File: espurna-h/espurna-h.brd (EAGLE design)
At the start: 50 x 50 mm, 55 parts, among them IC1 AMS1117-3.3, IC2 ESP-12-SMD, IC4 HLW8012

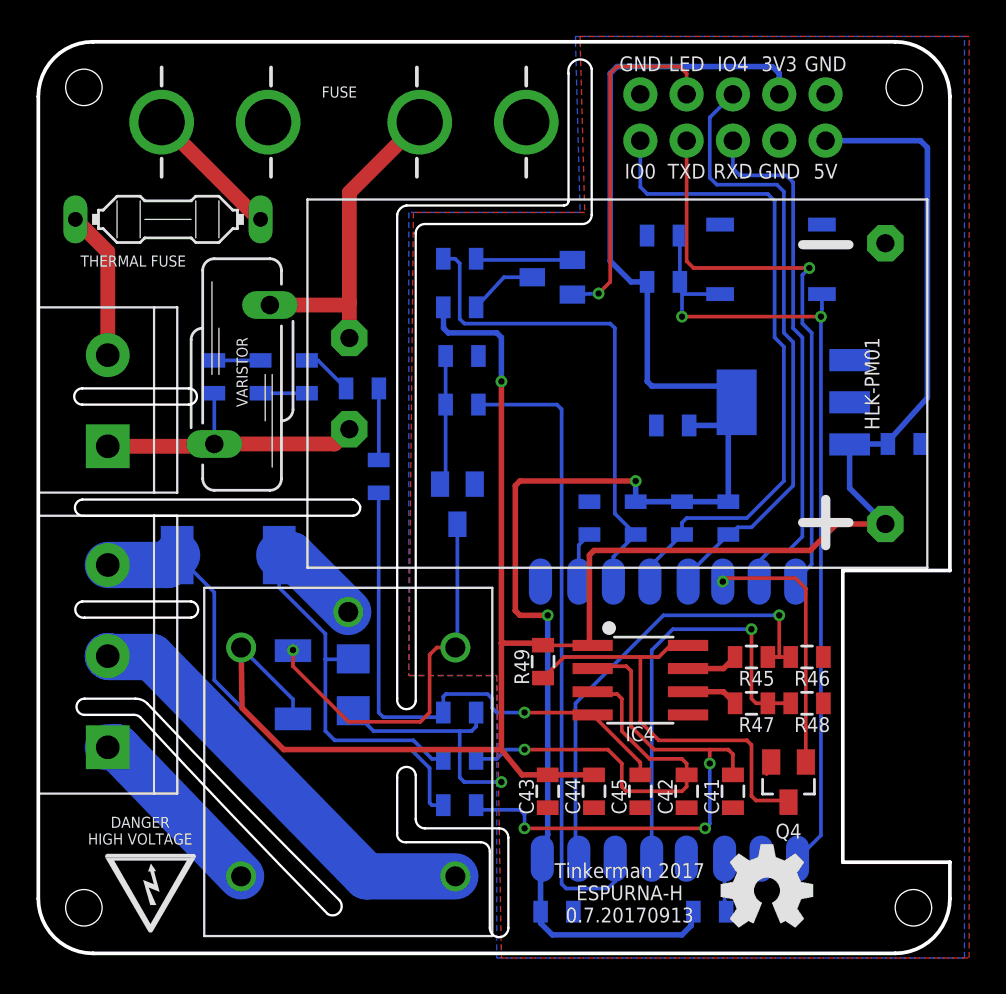
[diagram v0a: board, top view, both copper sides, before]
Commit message: Version 0.7.20170913
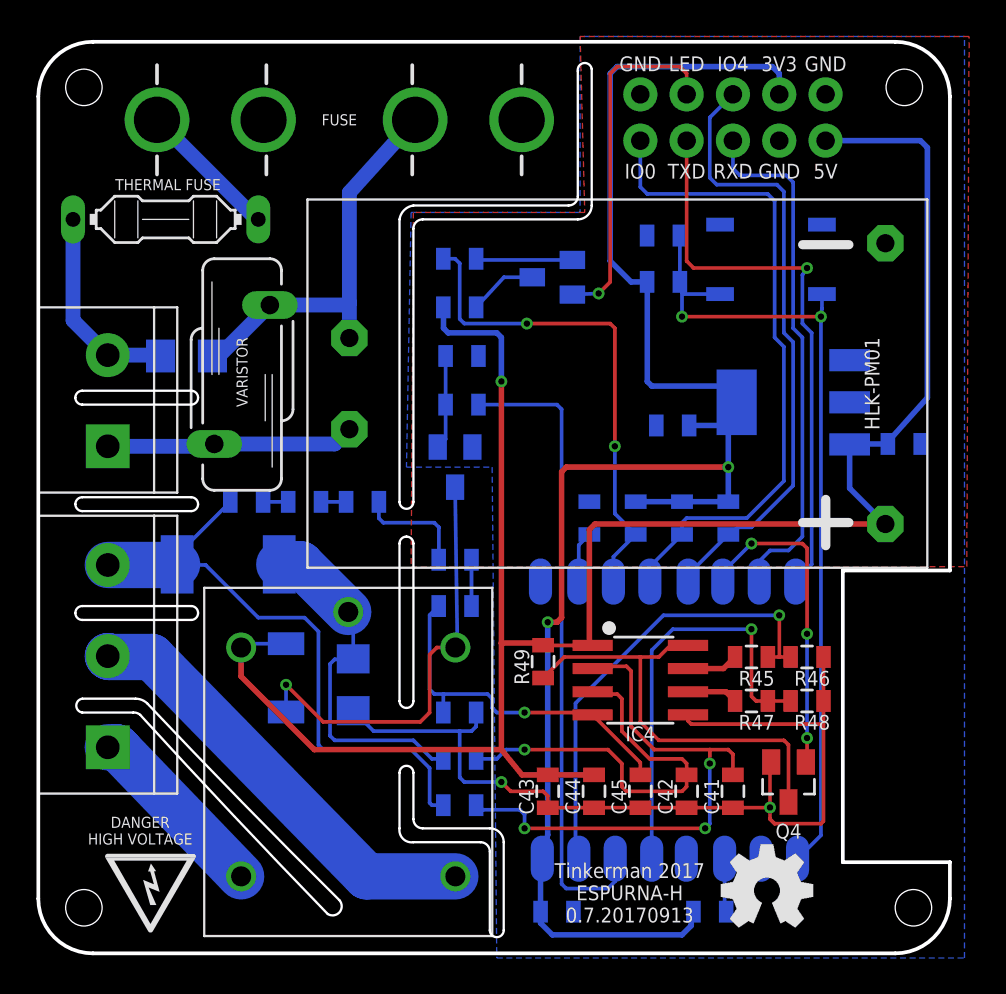
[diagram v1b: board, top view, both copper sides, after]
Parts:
- removed R1: 0.001R, xose:2512
- added R41: 0.001R, xose:2512
- added V11: S10K250, xose:S10K250
- R11: value S10K250 -> 0R; device xose:S10K250 -> xose:1206
- R42: value 0 -> 0R
- moved R54 10.7 mm to (22.9, 21.6)
- moved R55 8.25 mm to (22.9, 19.1), turned to 0 degrees
- moved R53 7.50 mm to (17.8, 24.8), turned to 0 degrees
- moved R52 7.27 mm to (14.6, 24.8), turned to 0 degrees
- moved R51 7.08 mm to (11.4, 24.8), turned to 0 degrees
- moved R11 3.21 mm to (8.13, 32.8), flipped to the bottom
- moved Q3 2.04 mm to (22.9, 26.7)
- moved D3 0.54 mm to (13.6, 15.1), turned to 90 degrees
- moved F2 0.28 mm to (16.5, 45.7)
- moved R47 0.13 mm to (39.1, 13.8)
- moved R48 0.13 mm to (42.2, 13.8)
- moved F1 0.13 mm to (6.99, 40.3)
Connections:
- removed net N$18: R52.1, R53.1
- removed net N$19: R51.2, R52.2
- new net N$15: R51.1, R52.2
- new net N$16: R52.1, R53.2
- net LINE_I: now also R11.2
- net LINE_L: now also R41.1; no longer R1.1
- net LINE_M: now also R41.2, R51.2; no longer R1.2
- net LINE_P: now also R11.1, V11.2; no longer R11.2
- net N$17: now also R53.1; no longer R53.2
- net NEUTRAL: now also V11.1; no longer R11.1, R51.1
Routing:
- net GND: track 13.8 -> 52.0 mm, vias 1 -> 2
- net V2P: track 30.2 -> 20.5 mm
- net LINE_M: track 28.2 -> 33.8 mm
- net LINE_L: track 24.8 -> 20.1 mm
- net LINE_P: track 17.9 -> 22.1 mm
- net N$17: track 2.78 -> 6.18 mm
- net GPIO5: track 14.4 -> 17.6 mm, vias 1 -> 3
- net LINE_I: track 8.18 -> 11.2 mm
- net NEUTRAL: track 16.4 -> 13.6 mm
- net 5V: track 114.3 -> 111.6 mm
- net N$4: track 21.4 -> 24.0 mm
- net N$19: track 2.54 -> 0.00 mm
- net N$18: track 2.54 -> 0.00 mm
- net N$5: track 7.15 -> 5.17 mm
- net N$6: track 3.93 -> 2.54 mm
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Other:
- outline, holes or cut-outs redrawn
